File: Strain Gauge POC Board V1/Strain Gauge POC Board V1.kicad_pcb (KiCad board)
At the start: 4 copper layers, 75.6 x 31.4 mm, 43 parts, among them J201 502352-0210, J202 502352-0210, U209 INA333xxDGK, U210 ADS1113IDGSR

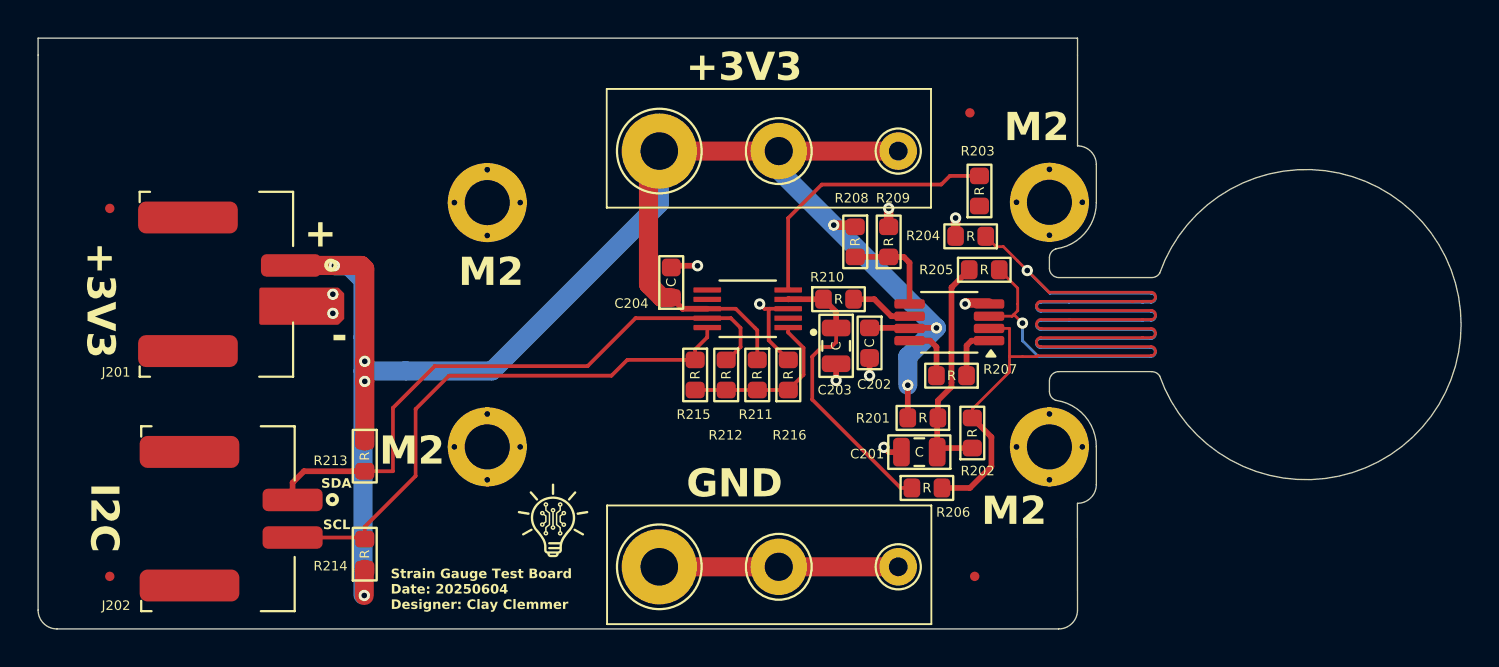
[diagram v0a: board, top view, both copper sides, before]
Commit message: almost finished first draft
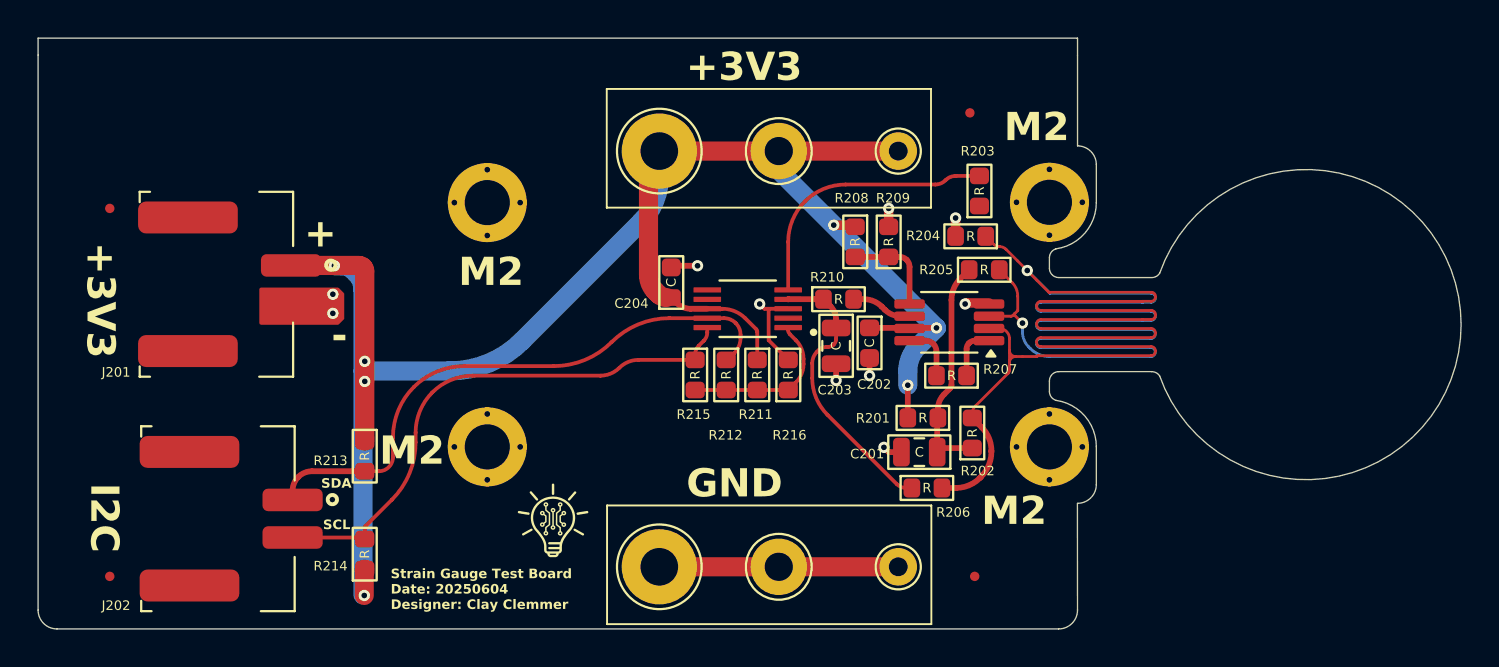
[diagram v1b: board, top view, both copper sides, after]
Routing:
- net +3V3a: track 106.4 -> 105.0 mm
- net Net-(U210-SDA): track 32.6 -> 31.2 mm
- net Net-(U210-SCL): track 29.8 -> 28.9 mm
- net Net-(C201-+): track 12.7 -> 12.1 mm
